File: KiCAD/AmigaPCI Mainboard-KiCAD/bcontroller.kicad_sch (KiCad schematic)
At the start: 17 parts, among them CN227 JTAG/SWD, J200 DISABLE AUTOBOOT, U6 XC95144XL-TQ144, U711 XC9572XL-VQ64

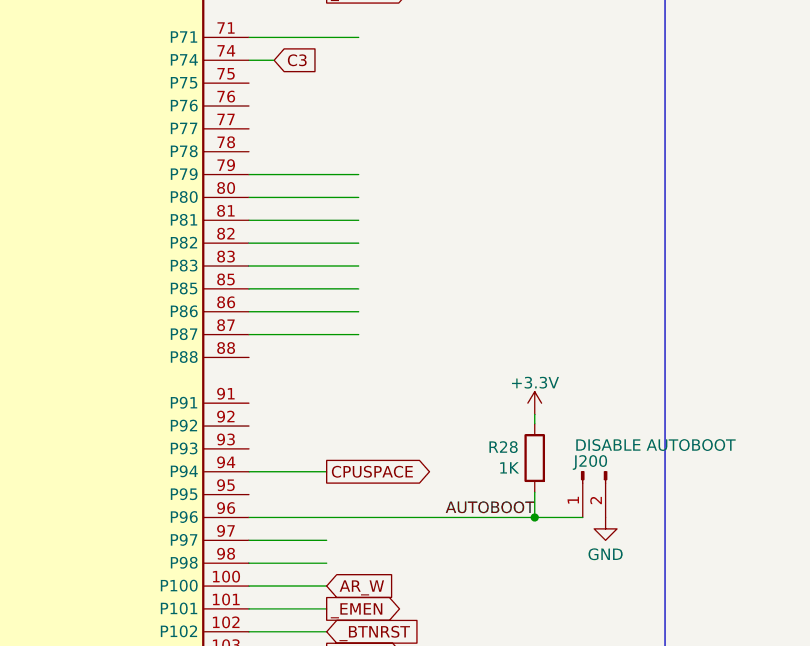
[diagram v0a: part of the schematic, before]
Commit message: Routing 23-DEC-2023
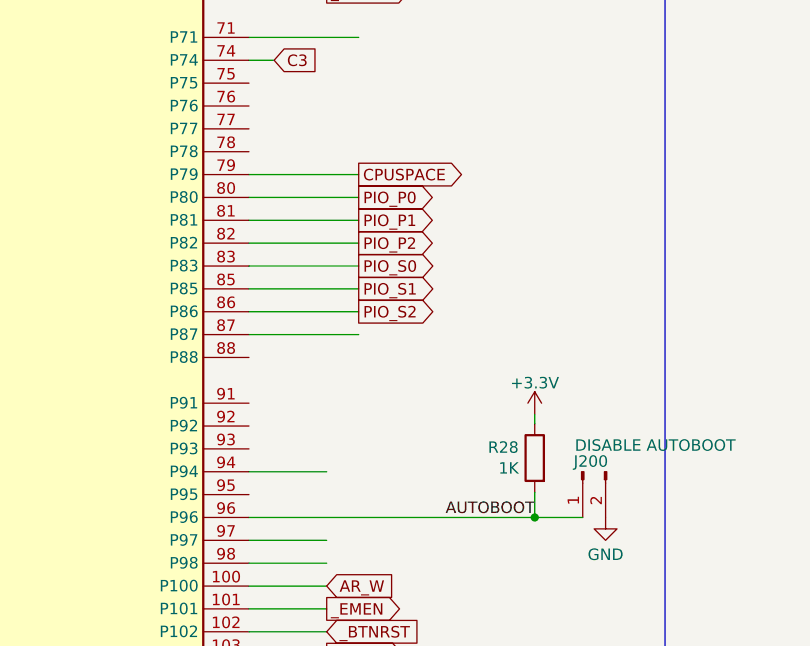
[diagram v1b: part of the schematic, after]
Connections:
- net CPUSPACE: now also U6.79 (P79); no longer U6.94 (P94)
- net PIO_P0: now reaches U6.80 (P80)
- net PIO_P1: now reaches U6.81 (P81)
- net PIO_P2: now reaches U6.82 (P82)
- net PIO_S0: now reaches U6.83 (P83)
- net PIO_S1: now reaches U6.85 (P85)
- net PIO_S2: now reaches U6.86 (P86)
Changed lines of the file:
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@@
+    )
+  )
+  (global_label "PIO_S2" (shape output) (at 191.008 174.752 0) (fields_autoplaced)
+    (effects (font (size 1.27 1.27)) (justify left))
+    (property "Intersheetrefs" "${INTERSHEET_REFS}" (at 200.5851 174.752 0)
+      (effects (font (size 1.27 1.27)) (justify left))
     )
   )
@@
     )
   )
+  (global_label "PIO_S0" (shape output) (at 191.008 169.672 0) (fields_autoplaced)
+    (effects (font (size 1.27 1.27)) (justify left))
+    (property "Intersheetrefs" "${INTERSHEET_REFS}" (at 200.5851 169.672 0)
+      (effects (font (size 1.27 1.27)) (justify left))
+    )
+  )
   (global_label "C3" (shape input) (at 181.61 146.812 0) (fields_autoplaced)
     (effects (font (size 1.27 1.27)) (justify left))
@@
     (property "Intersheetrefs" "${INTERSHEET_REFS}" (at 98.0895 192.532 0)
       (effects (font (size 1.27 1.27)) (justify right))
+    )
+  )
+  (global_label "PIO_P0" (shape output) (at 191.008 162.052 0) (fields_autoplaced)
+    (effects (font (size 1.27 1.27)) (justify left))
+    (property "Intersheetrefs" "${INTERSHEET_REFS}" (at 200.6456 162.052 0)
+      (effects (font (size 1.27 1.27)) (justify left))
     )
   )
@@
     )
   )
+  (global_label "PIO_S1" (shape output) (at 191.008 172.212 0) (fields_autoplaced)
+    (effects (font (size 1.27 1.27)) (justify left))
+    (property "Intersheetrefs" "${INTERSHEET_REFS}" (at 200.5851 172.212 0)
+      (effects (font (size 1.27 1.27)) (justify left))
+    )
+  )
   (global_label "_BEN" (shape output) (at 187.452 98.552 0) (fields_autoplaced)
     (effects (font (size 1.27 1.27)) (justify left))
@@
     )
   )
-  (global_label "CPUSPACE" (shape output) (at 187.452 192.532 0) (fields_autoplaced)
-    (effects (font (size 1.27 1.27)) (justify left))
-    (property "Intersheetrefs" "${INTERSHEET_REFS}" (at 200.2154 192.532 0)
+  (global_label "CPUSPACE" (shape output) (at 191.008 159.512 0) (fields_autoplaced)
+    (effects (font (size 1.27 1.27)) (justify left))
+    (property "Intersheetrefs" "${INTERSHEET_REFS}" (at 203.7714 159.512 0)
       (effects (font (size 1.27 1.27)) (justify left))
     )
@@
     )
   )
+  (global_label "PIO_P1" (shape output) (at 191.008 164.592 0) (fields_autoplaced)
+    (effects (font (size 1.27 1.27)) (justify left))
+    (property "Intersheetrefs" "${INTERSHEET_REFS}" (at 200.6456 164.592 0)
+      (effects (font (size 1.27 1.27)) (justify left))
+    )
+  )
   (global_label "_RTCWR" (shape output) (at 187.452 93.472 0) (fields_autoplaced)
     (effects (font (size 1.27 1.27)) (justify left))
@@
     )
   )
+  (global_label "PIO_P2" (shape output) (at 191.008 167.132 0) (fields_autoplaced)
+    (effects (font (size 1.27 1.27)) (justify left))
+    (property "Intersheetrefs" "${INTERSHEET_REFS}" (at 200.6456 167.132 0)
+      (effects (font (size 1.27 1.27)) (justify left))
+    )
+  )
